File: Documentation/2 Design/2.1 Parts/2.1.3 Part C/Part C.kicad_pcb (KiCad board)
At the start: 2 copper layers, 50 x 50 mm, 0 parts

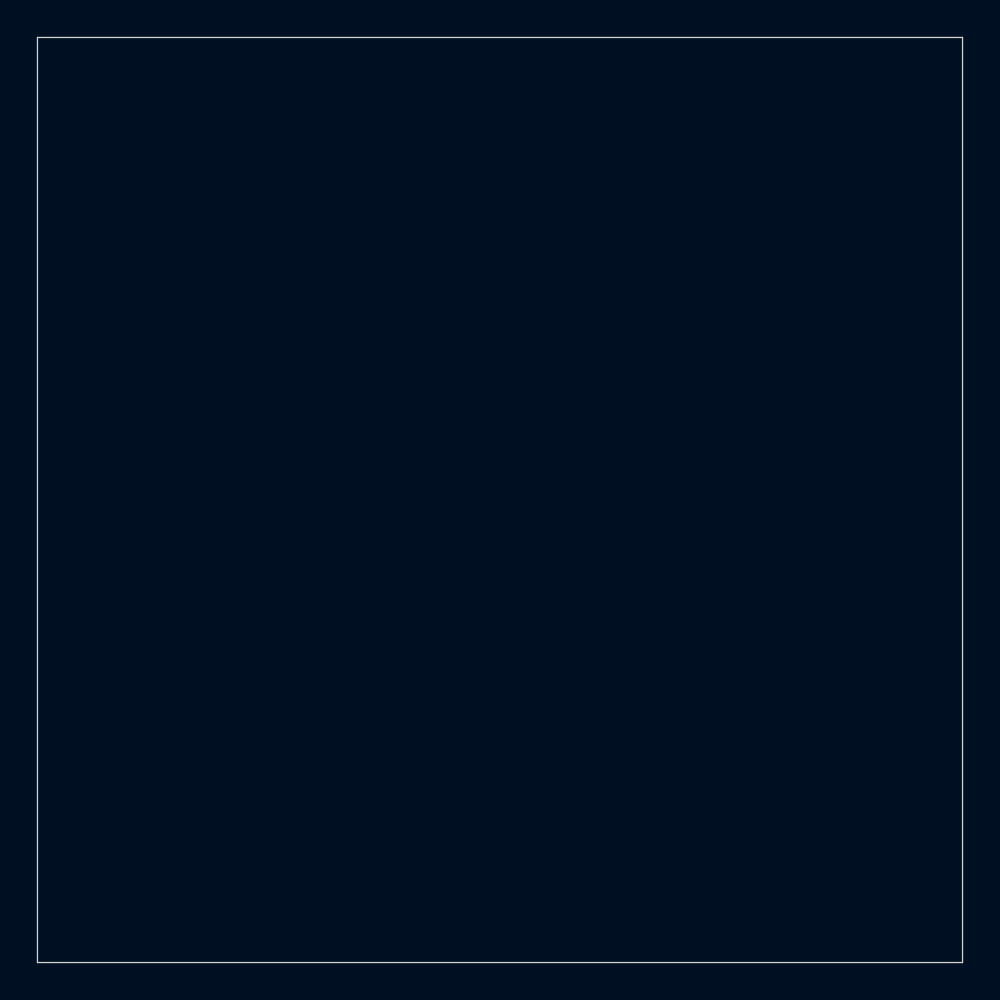
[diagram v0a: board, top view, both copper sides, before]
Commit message: Added extensions, plugins, some project documentation, demos of features
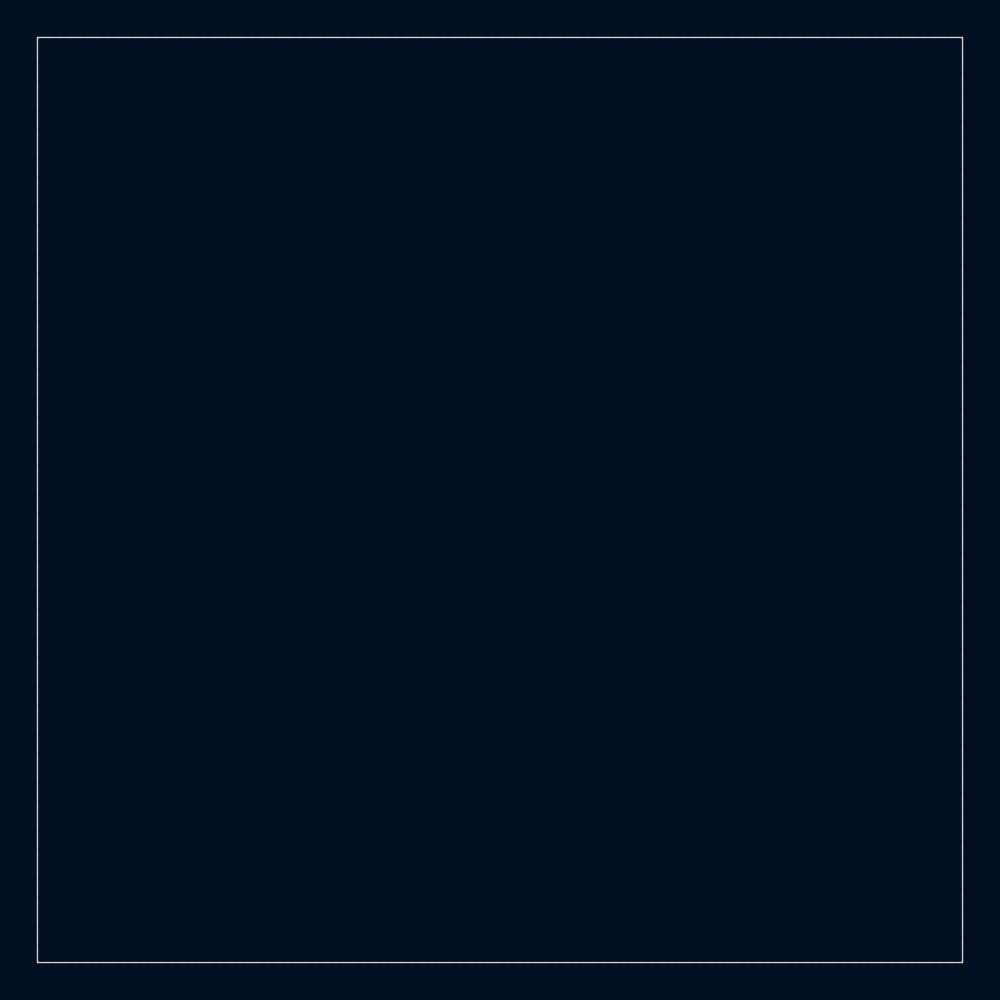
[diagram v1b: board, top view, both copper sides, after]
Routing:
- added copper zone on F.Cu, net (none)
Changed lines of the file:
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@@
 		(layer "Edge.Cuts")
+	)
+	(zone
+		(net 0)
+		(net_name "")
+		(layer "F.Cu")
+		(hatch edge 0.5)
+		(connect_pads
+			(clearance 0.5)
+		)
+		(min_thickness 0.25)
+		(filled_areas_thickness no)
+		(fill yes
+			(thermal_gap 0.5)
+			(thermal_bridge_width 0.5)
+			(island_removal_mode 1)
+			(island_area_min 10)
+		)
+		(polygon
+			(pts
+				(xy 125 75) (xy 175 75) (xy 175 125) (xy 125 125)
+			)
+		)
 	)
 	(embedded_fonts no)
